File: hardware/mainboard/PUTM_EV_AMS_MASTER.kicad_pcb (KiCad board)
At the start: 4 copper layers, 60 x 100 mm, 172 parts, among them IC3 BQ79600PWRQ1, IC6 AMC3330DWER, IC7 AMC3330DWER, IC8 ADC 24bit, IC9 LTC1799, J1 Conn_02x10_Odd_Even, J10 M300-MV10345M1, J2 XIAO ESP32S3 Sense, J3 Conn_02x04_Odd_Even, J4 FTSH-107-01-L-D-K, J5 M80-51004XX, J7 M300-MV10345M1, J8 M80-51004XX, Q6 2N7002, Q8 2N7002, Q9 2N7002, T1 SM91502ALE, U1 MAX40200AUK, U10 STM32H573RITx, U3 74AUP1G32

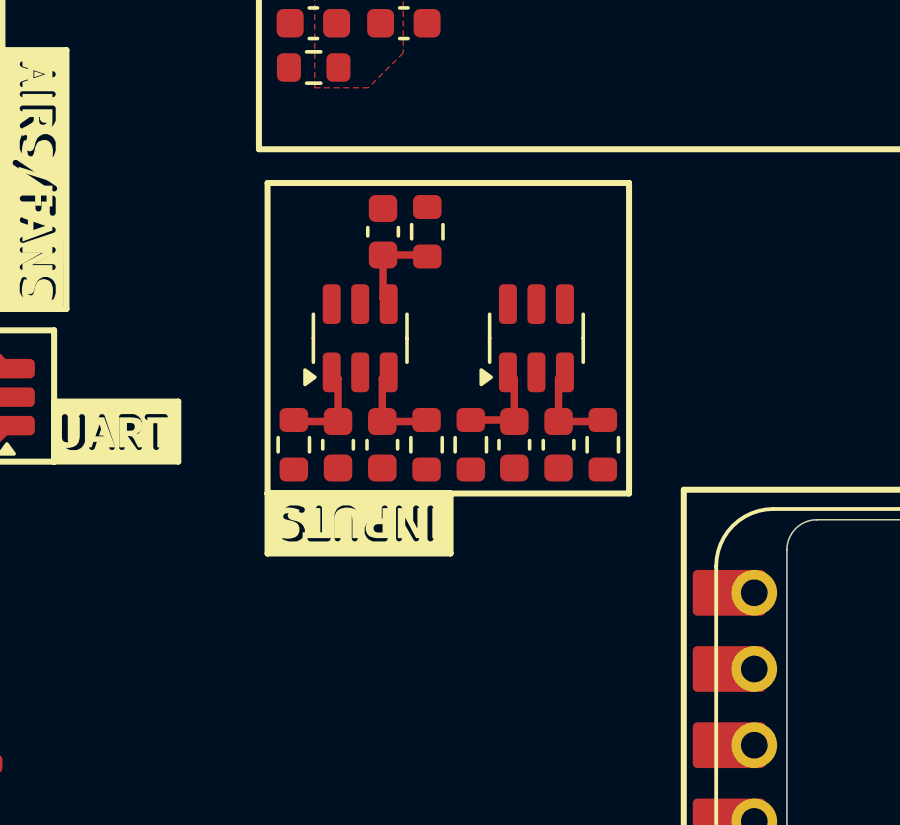
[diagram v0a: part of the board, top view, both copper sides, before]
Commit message: minifix2
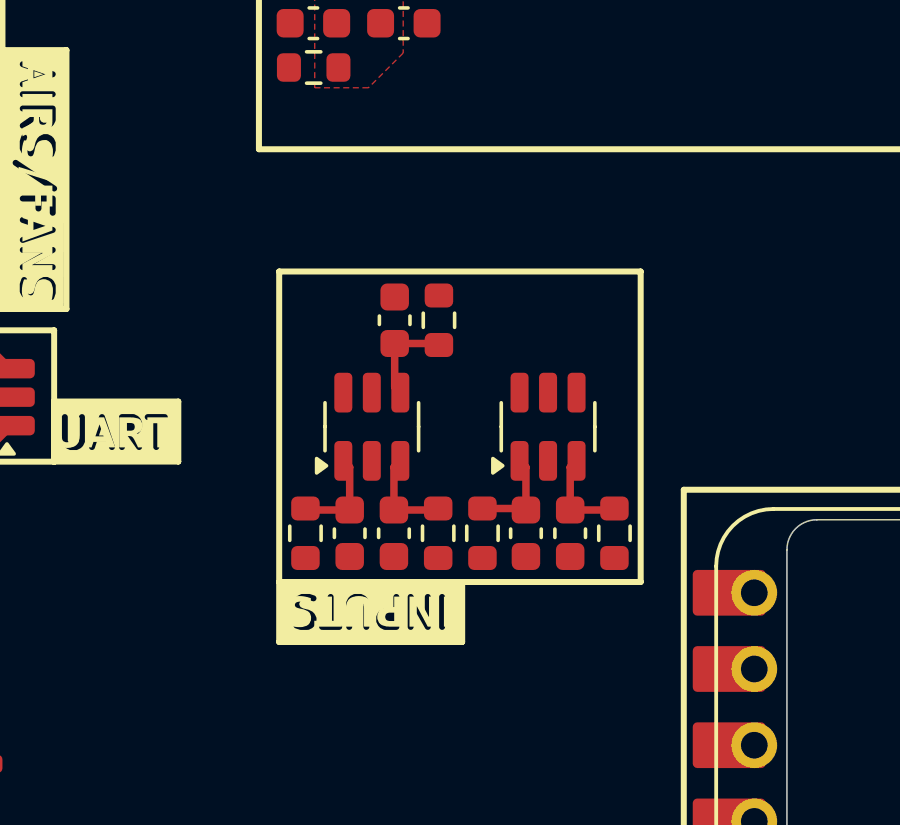
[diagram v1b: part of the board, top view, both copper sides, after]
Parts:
- moved C101 2.98 mm to (129.3, 126.7)
- moved C102 2.98 mm to (130.8, 126.7)
- moved C103 2.98 mm to (123.4, 126.7)
- moved C104 2.98 mm to (124.9, 126.7)
- moved C105 2.98 mm to (124.9, 119.5)
- moved R21 2.98 mm to (122.0, 126.7)
- moved R25 2.98 mm to (126.4, 126.7)
- moved R26 2.98 mm to (126.4, 119.5)
- moved R17 2.98 mm to (127.8, 126.7)
- moved R20 2.98 mm to (132.2, 126.7)
- moved D25 2.98 mm to (124.2, 123.1)
- moved D26 2.98 mm to (130.0, 123.1)
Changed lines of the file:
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@@
 	(footprint "Capacitor_SMD:C_0603_1608Metric"
 		(layer "F.Cu")
-		(at 124.5125 123.7 90)
+		(at 124.9 126.65 90)
 		(descr "Capacitor SMD 0603 (1608 Metric), square (rectangular) end terminal, IPC_7351 nominal, (Body size source: IPC-SM-782 page 76, https://www.pcb-3d.com/wordpress/wp-content/uploads/ipc-sm-782a_amendment_1_and_2.pdf), generated with kicad-footprint-generator")
 		(tags "capacitor")
@@
 	(footprint "Package_TO_SOT_SMD:SOT-23-6"
 		(layer "F.Cu")
-		(at 129.65 120.15 90)
+		(at 130.0375 123.1 90)
 		(descr "SOT, 6 Pin (JEDEC MO-178 Var AB https://www.jedec.org/document_search?search_api_views_fulltext=MO-178), generated with kicad-footprint-generator ipc_gullwing_generator.py")
 		(tags "SOT TO_SOT_SMD")
@@
 	(footprint "Resistor_SMD:R_0603_1608Metric"
 		(layer "F.Cu")
-		(at 131.8625 123.7 -90)
+		(at 132.25 126.65 -90)
 		(descr "Resistor SMD 0603 (1608 Metric), square (rectangular) end terminal, IPC_7351 nominal, (Body size source: IPC-SM-782 page 72, https://www.pcb-3d.com/wordpress/wp-content/uploads/ipc-sm-782a_amendment_1_and_2.pdf), generated with kicad-footprint-generator")
 		(tags "resistor")
@@
 	(footprint "Capacitor_SMD:C_0603_1608Metric"
 		(layer "F.Cu")
-		(at 124.5375 116.6 -90)
+		(at 124.925 119.55 -90)
 		(descr "Capacitor SMD 0603 (1608 Metric), square (rectangular) end terminal, IPC_7351 nominal, (Body size source: IPC-SM-782 page 76, https://www.pcb-3d.com/wordpress/wp-content/uploads/ipc-sm-782a_amendment_1_and_2.pdf), generated with kicad-footprint-generator")
 		(tags "capacitor")
@@
 	(footprint "Capacitor_SMD:C_0603_1608Metric"
 		(layer "F.Cu")
-		(at 123.0375 123.7 90)
+		(at 123.425 126.65 90)
 		(descr "Capacitor SMD 0603 (1608 Metric), square (rectangular) end terminal, IPC_7351 nominal, (Body size source: IPC-SM-782 page 76, https://www.pcb-3d.com/wordpress/wp-content/uploads/ipc-sm-782a_amendment_1_and_2.pdf), generated with kicad-footprint-generator")
 		(tags "capacitor")
@@
 	(footprint "Package_TO_SOT_SMD:SOT-23-6"
 		(layer "F.Cu")
-		(at 123.775 120.15 90)
+		(at 124.1625 123.1 90)
 		(descr "SOT, 6 Pin (JEDEC MO-178 Var AB https://www.jedec.org/document_search?search_api_views_fulltext=MO-178), generated with kicad-footprint-generator ipc_gullwing_generator.py")
 		(tags "SOT TO_SOT_SMD")
@@
 	(footprint "Resistor_SMD:R_0603_1608Metric"
 		(layer "F.Cu")
-		(at 121.5625 123.7 -90)
+		(at 121.95 126.65 -90)
 		(descr "Resistor SMD 0603 (1608 Metric), square (rectangular) end terminal, IPC_7351 nominal, (Body size source: IPC-SM-782 page 72, https://www.pcb-3d.com/wordpress/wp-content/uploads/ipc-sm-782a_amendment_1_and_2.pdf), generated with kicad-footprint-generator")
 		(tags "resistor")
@@
 	(footprint "Resistor_SMD:R_0603_1608Metric"
 		(layer "F.Cu")
-		(at 126.0125 116.6 90)
+		(at 126.4 119.55 90)
 		(descr "Resistor SMD 0603 (1608 Metric), square (rectangular) end terminal, IPC_7351 nominal, (Body size source: IPC-SM-782 page 72, https://www.pcb-3d.com/wordpress/wp-content/uploads/ipc-sm-782a_amendment_1_and_2.pdf), generated with kicad-footprint-generator")
 		(tags "resistor")
@@
 	(footprint "Capacitor_SMD:C_0603_1608Metric"
 		(layer "F.Cu")
-		(at 130.3875 123.7 90)
+		(at 130.775 126.65 90)
 		(descr "Capacitor SMD 0603 (1608 Metric), square (rectangular) end terminal, IPC_7351 nominal, (Body size source: IPC-SM-782 page 76, https://www.pcb-3d.com/wordpress/wp-content/uploads/ipc-sm-782a_amendment_1_and_2.pdf), generated with kicad-footprint-generator")
 		(tags "capacitor")
@@
 	(footprint "Capacitor_SMD:C_0603_1608Metric"
 		(layer "F.Cu")
-		(at 128.9125 123.7 90)
+		(at 129.3 126.65 90)
 		(descr "Capacitor SMD 0603 (1608 Metric), square (rectangular) end terminal, IPC_7351 nominal, (Body size source: IPC-SM-782 page 76, https://www.pcb-3d.com/wordpress/wp-content/uploads/ipc-sm-782a_amendment_1_and_2.pdf), generated with kicad-footprint-generator")
 		(tags "capacitor")
@@
 	(footprint "Resistor_SMD:R_0603_1608Metric"
 		(layer "F.Cu")
-		(at 125.9875 123.7 -90)
+		(at 126.375 126.65 -90)
 		(descr "Resistor SMD 0603 (1608 Metric), square (rectangular) end terminal, IPC_7351 nominal, (Body size source: IPC-SM-782 page 72, https://www.pcb-3d.com/wordpress/wp-content/uploads/ipc-sm-782a_amendment_1_and_2.pdf), generated with kicad-footprint-generator")
 		(tags "resistor")
@@
 	(footprint "Resistor_SMD:R_0603_1608Metric"
 		(layer "F.Cu")
-		(at 127.4625 123.7 -90)
+		(at 127.85 126.65 -90)
 		(descr "Resistor SMD 0603 (1608 Metric), square (rectangular) end terminal, IPC_7351 nominal, (Body size source: IPC-SM-782 page 72, https://www.pcb-3d.com/wordpress/wp-content/uploads/ipc-sm-782a_amendment_1_and_2.pdf), generated with kicad-footprint-generator")
 		(tags "resistor")
@@
 	)
 	(gr_rect
-		(start 120.6875 114.975)
-		(end 132.7375 125.325)
+		(start 121.075 117.925)
+		(end 133.125 128.275)
 		(stroke
 			(width 0.2)
@@
 	)
 	(gr_rect
-		(start 120.6875 125.325)
-		(end 126.7875 127.325)
+		(start 121.075 128.275)
+		(end 127.175 130.275)
 		(stroke
 			(width 0.2)
@@
 	)
 	(gr_text "INPUTS"
-		(at 123.7125 126.275 180)
+		(at 124.1 129.225 180)
 		(layer "F.SilkS" knockout)
 		(effects
@@
 	)
 	(segment
-		(start 124.5125 122.925)
-		(end 125.9375 122.925)
+		(start 124.9 125.875)
+		(end 126.325 125.875)
 		(width 0.25)
 		(layer "F.Cu")
@@
 	)
 	(segment
-		(start 124.5125 122.925)
-		(end 124.5125 121.5)
+		(start 124.9 125.875)
+		(end 124.9 124.45)
 		(width 0.25)
 		(layer "F.Cu")
@@
 	)
 	(segment
-		(start 124.5125 121.5)
-		(end 124.725 121.2875)
+		(start 124.9 124.45)
+		(end 125.1125 124.2375)
 		(width 0.25)
 		(layer "F.Cu")
@@
 	)
 	(segment
-		(start 128.8625 122.875)
-		(end 128.9125 122.925)
+		(start 129.25 125.825)
+		(end 129.3 125.875)
 		(width 0.25)
 		(layer "F.Cu")
@@
 	)
 	(segment
-		(start 127.4625 122.875)
-		(end 128.8625 122.875)
+		(start 127.85 125.825)
+		(end 129.25 125.825)
 		(width 0.25)
 		(layer "F.Cu")
@@
 	)
 	(segment
-		(start 128.9125 122.925)
-		(end 128.9125 121.5)
+		(start 129.3 125.875)
+		(end 129.3 124.45)
 		(width 0.25)
 		(layer "F.Cu")
@@
 	)
 	(segment
-		(start 128.9125 121.5)
-		(end 128.7 121.2875)
+		(start 129.3 124.45)
+		(end 129.0875 124.2375)
 		(width 0.25)
 		(layer "F.Cu")
@@
 	)
 	(segment
-		(start 130.3875 121.5)
-		(end 130.6 121.2875)
+		(start 130.775 124.45)
+		(end 130.9875 124.2375)
 		(width 0.25)
 		(layer "F.Cu")
@@
 	)
 	(segment
-		(start 130.3875 122.925)
-		(end 131.8125 122.925)
+		(start 130.775 125.875)
+		(end 132.2 125.875)
 		(width 0.25)
 		(layer "F.Cu")
@@
 	)
 	(segment
-		(start 130.3875 122.925)
-		(end 130.3875 121.5)
+		(start 130.775 125.875)
+		(end 130.775 124.45)
 		(width 0.25)
 		(layer "F.Cu")
@@
 	)
 	(segment
-		(start 131.8125 122.925)
-		(end 131.8625 122.875)
+		(start 132.2 125.875)
+		(end 132.25 125.825)
 		(width 0.25)
 		(layer "F.Cu")
@@
 	)
 	(segment
-		(start 131.8625 124.375)
-		(end 131.9125 124.325)
+		(start 132.25 127.325)
+		(end 132.3 127.275)
 		(width 0.1275)
 		(layer "F.Cu")
@@
 	)
 	(segment
-		(start 124.5375 117.375)
-		(end 124.5375 118.825)
+		(start 124.925 120.325)
+		(end 124.925 121.775)
 		(width 0.25)
 		(layer "F.Cu")
@@
 	)
 	(segment
-		(start 124.5375 117.375)
-		(end 125.9625 117.375)
+		(start 124.925 120.325)
+		(end 126.35 120.325)
 		(width 0.25)
 		(layer "F.Cu")
@@
 	)
 	(segment
-		(start 124.5375 118.825)
-		(end 124.725 119.0125)
+		(start 124.925 121.775)
+		(end 125.1125 121.9625)
 		(width 0.25)
 		(layer "F.Cu")
@@
 	)
 	(segment
-		(start 123.0375 122.925)
-		(end 123.0375 121.5)
+		(start 123.425 125.875)
+		(end 123.425 124.45)
 		(width 0.25)
 		(layer "F.Cu")
@@
 	)
 	(segment
-		(start 123.0375 122.925)
-		(end 121.6125 122.925)
+		(start 123.425 125.875)
+		(end 122 125.875)
 		(width 0.25)
 		(layer "F.Cu")
@@
 	)
 	(segment
-		(start 123.0375 121.5)
-		(end 122.825 121.2875)
+		(start 123.425 124.45)
+		(end 123.2125 124.2375)
 		(width 0.25)
 		(layer "F.Cu")
@@
 	)
 	(segment
-		(start 127.5625 124.375)
-		(end 127.5125 124.325)
+		(start 127.95 127.325)
+		(end 127.9 127.275)
 		(width 0.1275)
 		(layer "F.Cu")
@@
 		(polygon
 			(pts
-				(xy 126.7875 127.325) (xy 126.7875 125.325) (xy 120.6875 125.325) (xy 120.6875 127.325)
+				(xy 127.175 130.275) (xy 127.175 128.275) (xy 121.075 128.275) (xy 121.075 130.275)
 			)
 		)
